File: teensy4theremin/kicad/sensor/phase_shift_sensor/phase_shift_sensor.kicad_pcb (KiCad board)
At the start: 2 copper layers, 59.7 x 22.9 mm, 15 parts, among them J1 SENSOR, J2 L_IN, J3 L_OUT, J4 ANT, U1 74AC86, U2 sp721

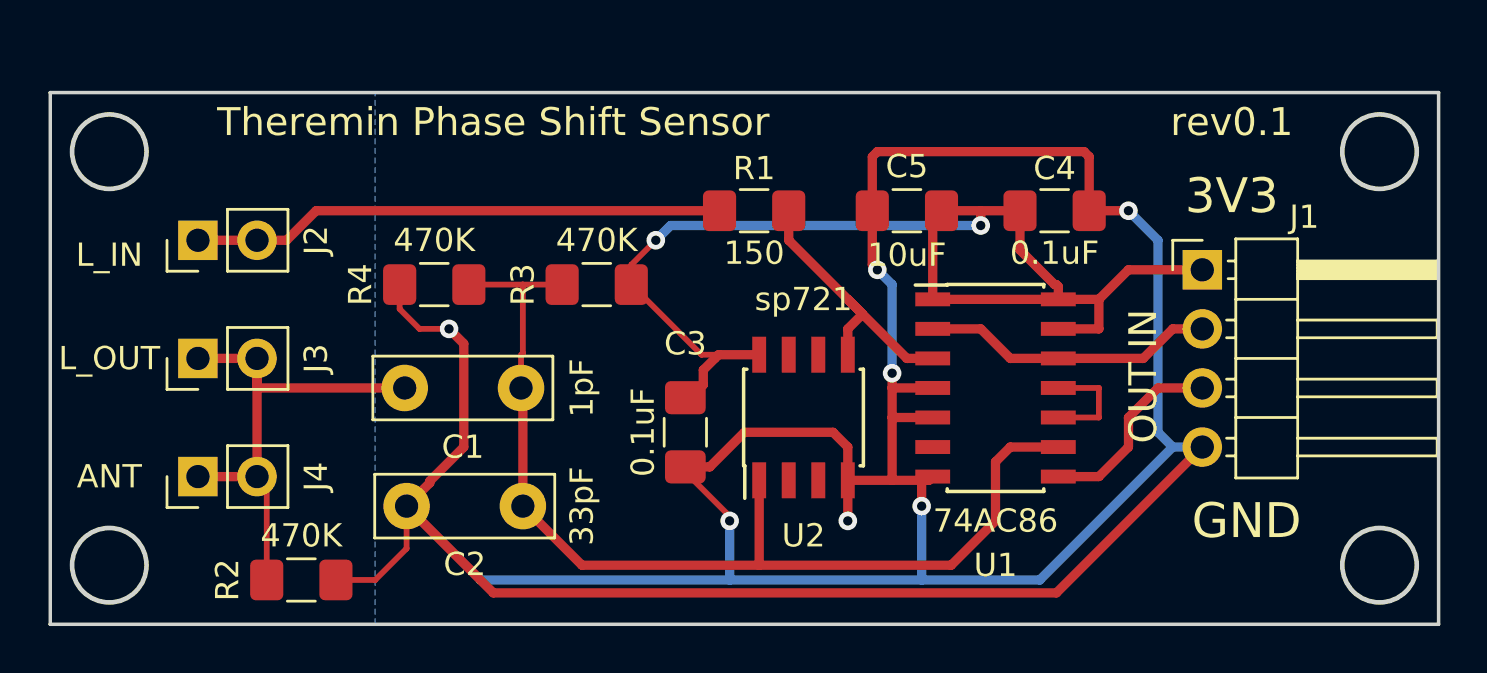
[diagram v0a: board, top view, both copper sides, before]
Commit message: update
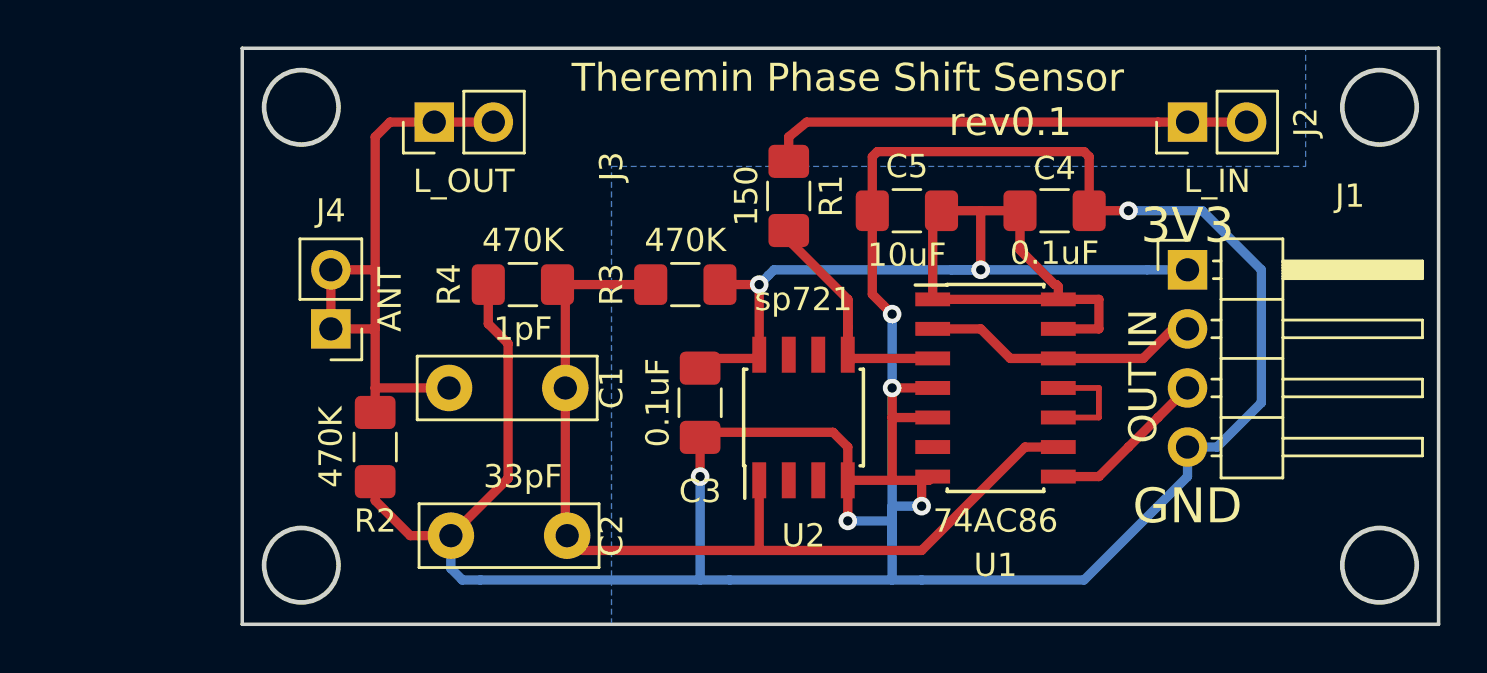
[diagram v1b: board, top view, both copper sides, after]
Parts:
- moved J2 42.8 mm to (139.1, 72.4)
- moved J3 14.4 mm to (106.7, 72.4)
- moved J4 8.54 mm to (102.2, 81.3), turned to 180 degrees
- moved R2 6.54 mm to (104.1, 86.4), turned to 90 degrees
- moved R3 3.81 mm to (117.5, 79.4)
- moved R4 3.81 mm to (110.5, 79.4)
- moved C2 2.29 mm to (112.4, 90.2)
- moved C1 1.91 mm to (107.3, 83.8)
- moved R1 1.62 mm to (121.9, 75.6), turned to 270 degrees
- moved C3 1.42 mm to (118.1, 84.5)
- moved J1 0.63 mm to (139.1, 78.7)
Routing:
- net GND: track 161.4 -> 136.1 mm, vias 7 -> 6
- net Net-(C1-Pad1): track 22.4 -> 26.7 mm
- net Net-(C1-Pad2): track 44.9 -> 41.3 mm
- net +3V3: track 55.4 -> 52.0 mm
- net Net-(J2-Pad1): track 23.0 -> 21.0 mm
- net /PWM_OUT: track 8.51 -> 7.13 mm
- net /REF_CLK: track 12.6 -> 12.0 mm
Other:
- board size 59.7 x 22.9 mm -> 51.4 x 24.8 mm
